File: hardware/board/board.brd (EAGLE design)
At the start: 47 x 50.5 mm, 7 parts, among them M1 WIRELESS-NRF24L01, X1 MAB7SH

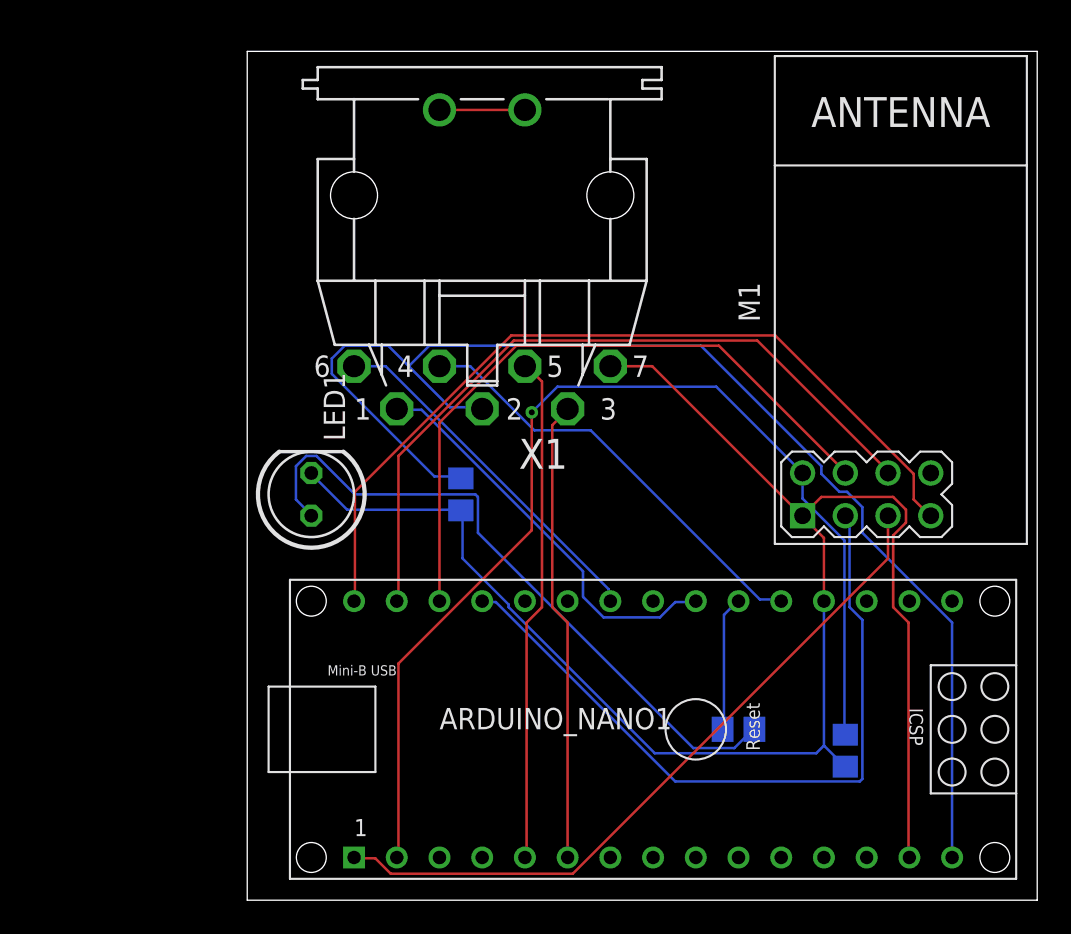
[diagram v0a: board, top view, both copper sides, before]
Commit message: fixed circuitboard
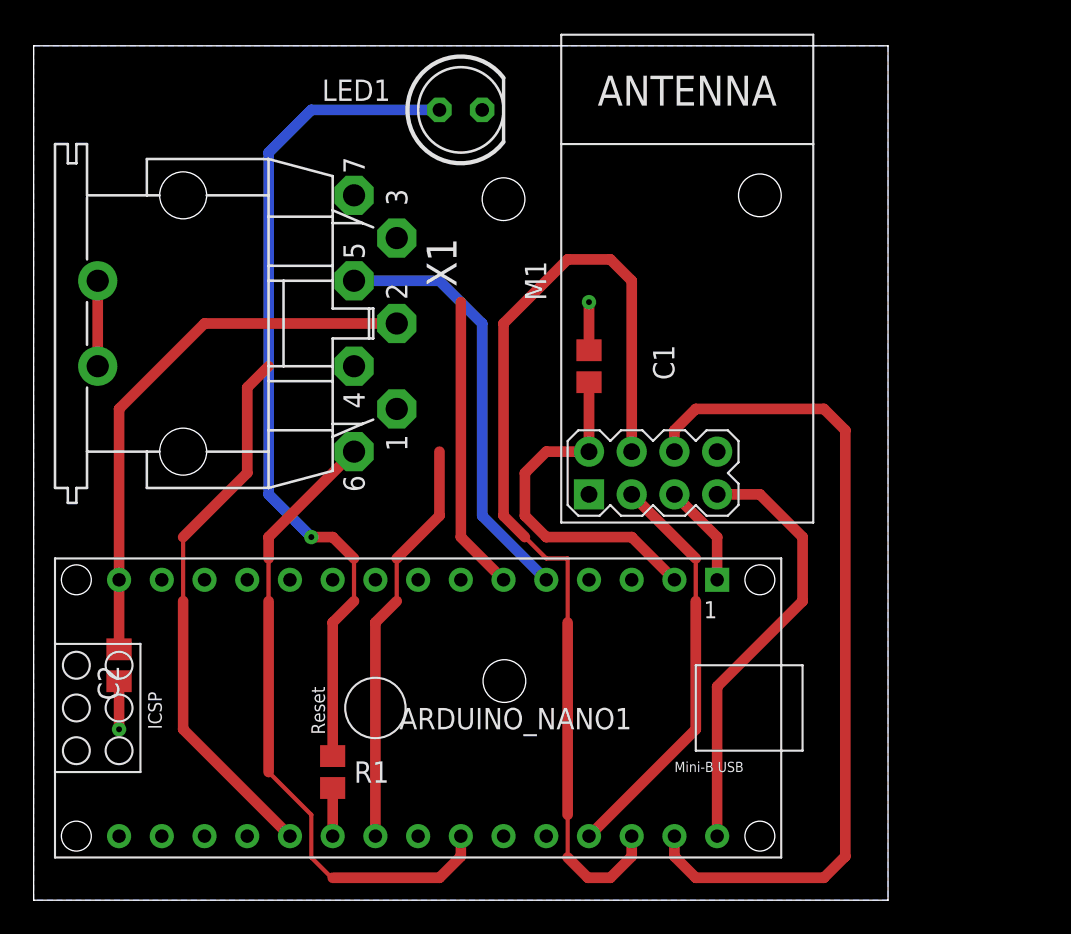
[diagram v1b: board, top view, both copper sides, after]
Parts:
- C1, C2: value 10 uF -> 22 uF
- moved C1 27.5 mm to (20.3, 34.3), flipped to the top, turned to 270 degrees
- moved LED1 24.5 mm to (12.7, 49.5), turned to 0 degrees
- moved R1 24.3 mm to (5.08, 10.2), flipped to the top, turned to 90 degrees
- moved C2 22.7 mm to (-7.62, 16.5), flipped to the top
- moved X1 19.3 mm to (-3.81, 36.8), turned to 270 degrees
- moved ARDUINO_NANO1 19.1 mm to (7.62, 14.0), turned to 180 degrees
- moved M1 12.8 mm to (26.7, 39.4)
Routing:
- net GND: track 98.7 -> 5.72 mm, vias 0 -> 2
- net VIN: track 76.8 -> 32.9 mm
- net 3V3: track 65.3 -> 21.5 mm, vias 1 -> 0
- net N$1: track 42.5 -> 6.13 mm
- net N$2: track 49.9 -> 26.0 mm
- net N$4: track 39.8 -> 60.0 mm
- net N$5: track 43.2 -> 24.5 mm
- net N$8: track 21.4 -> 38.4 mm
- net N$6: track 39.7 -> 50.5 mm, vias 0 -> 1
- net N$13: track 27.4 -> 17.6 mm
- net N$12: track 26.1 -> 32.7 mm
- net N$3: track 43.9 -> 50.2 mm
- net N$7: track 8.03 -> 2.86 mm
- net N$11: track 30.1 -> 25.5 mm
- added copper zone on layer 16, net GND
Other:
- board size 47 x 50.5 mm -> 50.8 x 50.8 mm
- board text added: "nanopi ptc rev 1.1"
